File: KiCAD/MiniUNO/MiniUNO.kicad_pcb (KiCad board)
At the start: 2 copper layers, 22 x 18 mm, 28 parts, among them IC1 AZ1117CR2-5.0TRG1, J1 USB_B_Micro, J2 Conn_01x11, J3 Conn_01x11, J4 Conn_01x07, Q1 FDN340P, Q2 PMV48XP, U1 ATmega32U4-A, Y1 830108288709

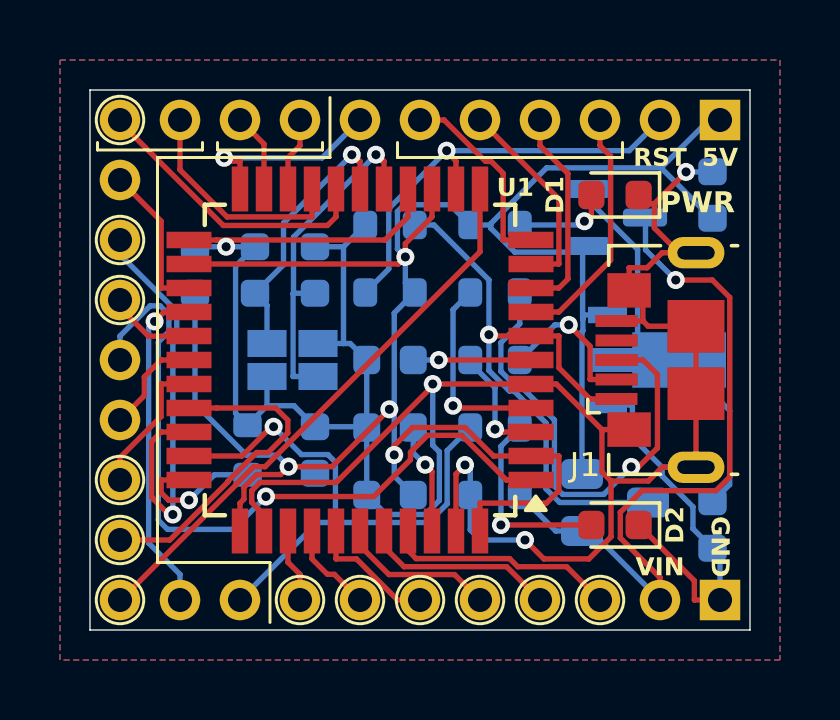
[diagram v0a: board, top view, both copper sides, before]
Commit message: Finalized design v1
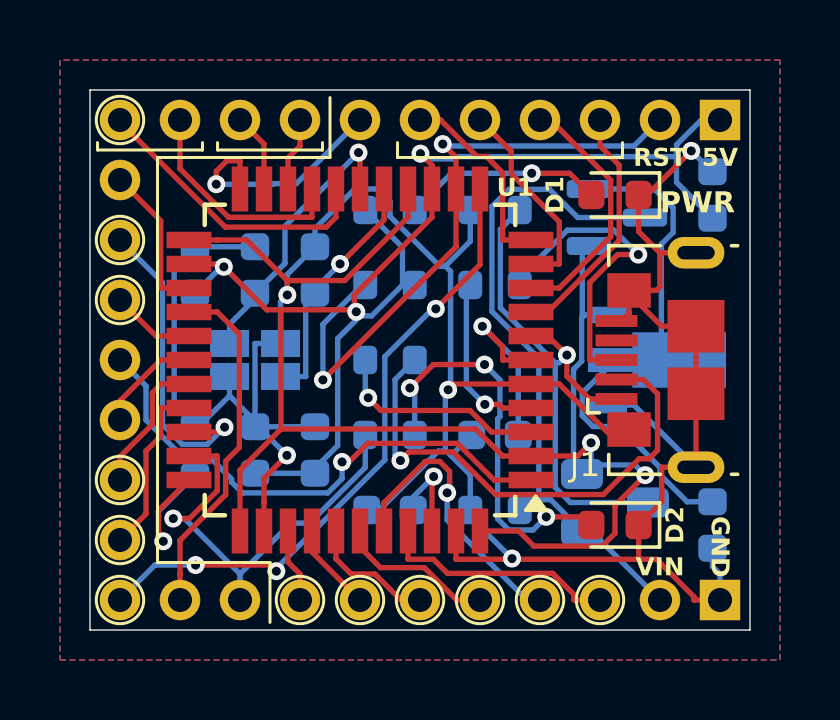
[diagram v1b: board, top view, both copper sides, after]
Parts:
- moved C6 4.30 mm to (4.50, 2.50)
- moved R5 3.54 mm to (1.00, -5.00)
- moved R7 3.54 mm to (4.50, -5.00)
- moved R6 3.51 mm to (1.00, 2.50)
- moved R2 3.50 mm to (1.00, 0.00)
- moved C5 2.92 mm to (-1.50, 3.00), turned to 90 degrees
- moved C7 2.75 mm to (1.00, 5.00)
- moved C4 2.00 mm to (-3.50, 3.00)
- moved R3 1.75 mm to (-5.50, 3.00)
- moved Y1 1.25 mm to (-3.50, 0.00)
- moved R8 0.50 mm to (4.50, 5.00)
- moved R1 0.25 mm to (4.50, -2.50)
- moved R4 0.25 mm to (1.00, -2.50)
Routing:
- net Net-(J1-D-): track 5.11 -> 17.6 mm
- net Net-(D2-A): track 6.52 -> 13.9 mm, vias 1 -> 3
- net D7: track 24.6 -> 17.8 mm
- net RESET: track 14.8 -> 21.3 mm, vias 1 -> 2
- net Net-(J1-D+): track 15.8 -> 10.7 mm
- net D10: track 11.0 -> 5.90 mm
- net Net-(IC1-IN): track 14.3 -> 18.8 mm
- net D13/USER_LED: track 18.9 -> 14.5 mm
- net D11: track 18.9 -> 22.8 mm, vias 0 -> 3
- net +5V: track 74.8 -> 78.7 mm, vias 4 -> 5
- net A4: track 6.46 -> 10.2 mm, vias 0 -> 1
- net D5: track 14.2 -> 10.6 mm
- net Net-(D1-A): track 3.18 -> 6.69 mm
- net D-: track 3.89 -> 7.20 mm
- net XTAL2: track 11.4 -> 8.17 mm
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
